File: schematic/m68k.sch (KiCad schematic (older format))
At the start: 45 parts, among them J1 Power, J2 CONN_01X03, J3 JTAG, J4 CONN_02X30, J5 I2C, J6 CONN_02X30, J7 CONN_01X02, J8 CONN_02X30, J9 CONN_01X03, SW1 SW_Push_Dual, U1 M68SEC000, U10 MCP23008, U2 AS6C8016, U3 LM1084IT-3.3/NOPB, U4 AT28BV64, U5 AT28BV64, U6 XC9572XL-VQ44, U7 MCP23017, U8 XO91-16, U9 XO91-50

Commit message: corrected footprints
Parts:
- J1: symbol Conn_01X04 -> CONN_01X04
- J2, J5, J9: symbol Conn_01X03 -> CONN_01X03
- J3: symbol Conn_01X06 -> CONN_01X06
- J4, J6, J8: symbol Conn_02X30 -> CONN_02X30
- J7: footprint Pin_Headers:Pin_Header_Straight_1x02 -> Pin_Headers:Pin_Header_Straight_1x02_Pitch2.54mm; symbol Conn_01X02 -> CONN_01X02
- U4, U5, U7: footprint SMD_Packages:SOIC-28 -> Housings_SOIC:SOIC-28W_7.5x17.9mm_Pitch1.27mm
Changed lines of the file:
@@
 LIBS:switches
 LIBS:m68k-cache
-EELAYER 26 0
+EELAYER 25 0
 EELAYER END
 $Descr A3 16535 11693
@@
 CLK_50MHz
 $Comp
-L Conn_01X06 J3
+L CONN_01X06 J3
 U 1 1 59881DD2
 P 4850 6750
@@
 $EndComp
 $Comp
-L Conn_01X03 J2
+L CONN_01X03 J2
 U 1 1 59883D86
 P 6150 6850
@@
 F 0 "U4" H 8200 2600 60  0000 C CNN
 F 1 "AT28BV64" H 8000 1100 60  0000 C CNN
-F 2 "SMD_Packages:SOIC-28" H 7950 1250 60  0001 C CNN
+F 2 "Housings_SOIC:SOIC-28W_7.5x17.9mm_Pitch1.27mm" H 7950 1250 60  0001 C CNN
 F 3 "" H 7950 1250 60  0001 C CNN
 	1    8000 1900
@@
 F 0 "U5" H 8200 4400 60  0000 C CNN
 F 1 "AT28BV64" H 8000 2900 60  0000 C CNN
-F 2 "SMD_Packages:SOIC-28" H 7950 3050 60  0001 C CNN
+F 2 "Housings_SOIC:SOIC-28W_7.5x17.9mm_Pitch1.27mm" H 7950 3050 60  0001 C CNN
 F 3 "" H 7950 3050 60  0001 C CNN
 	1    8000 3700
@@
 $EndComp
 $Comp
-L Conn_01X04 J1
+L CONN_01X04 J1
 U 1 1 5989E226
 P 3850 6850
@@
 F 0 "U7" H 12900 6075 50  0000 R CNN
 F 1 "MCP23017" H 12900 6000 50  0000 R CNN
-F 2 "SMD_Packages:SOIC-28" H 13050 4100 50  0001 L CNN
+F 2 "Housings_SOIC:SOIC-28W_7.5x17.9mm_Pitch1.27mm" H 13050 4100 50  0001 L CNN
 F 3 "" H 13250 6050 50  0001 C CNN
 	1    13000 5050
@@
 NoConn ~ 3250 1400
 $Comp
-L Conn_01X03 J5
+L CONN_01X03 J5
 U 1 1 598BE077
 P 2750 6800
@@
 Connection ~ 1950 6800
 $Comp
-L Conn_02X30 J4
+L CONN_02X30 J4
 U 1 1 598BF124
 P 7600 8900
@@
 ~HALT
 $Comp
-L Conn_01X03 J9
+L CONN_01X03 J9
 U 1 1 599050EF
 P 12300 3050
@@
 ~RESET
 $Comp
-L Conn_01X02 J7
+L CONN_01X02 J7
 U 1 1 59934E94
 P 9550 1700
 F 0 "J7" H 9550 1850 50  0000 C CNN
 F 1 "CONN_01X02" V 9650 1700 50  0000 C CNN
-F 2 "Pin_Headers:Pin_Header_Straight_1x02" H 9550 1700 50  0001 C CNN
+F 2 "Pin_Headers:Pin_Header_Straight_1x02_Pitch2.54mm" H 9550 1700 50  0001 C CNN
 F 3 "" H 9550 1700 50  0001 C CNN
 	1    9550 1700
@@
 ~IPL2
 $Comp
-L Conn_02X30 J6
+L CONN_02X30 J6
 U 1 1 5997FD38
 P 8750 8900
@@
 ~IPL2
 $Comp
-L Conn_02X30 J8
+L CONN_02X30 J8
 U 1 1 5997FDC7
 P 9900 8900

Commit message: bla
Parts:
- U3: footprint TO_SOT_Packages_THT:TO-220_Vertical -> TO_SOT_Packages_THT:TO-220_Horizontal
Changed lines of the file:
@@
 LIBS:switches
 LIBS:m68k-cache
-EELAYER 25 0
+EELAYER 26 0
 EELAYER END
 $Descr A3 16535 11693
@@
 F 0 "U3" H 5100 4600 50  0000 C CNN
 F 1 "LM1084IT-3.3/NOPB" H 4600 5000 50  0000 L CNN
-F 2 "TO_SOT_Packages_THT:TO-220_Vertical" H 4900 4900 50  0001 C CIN
+F 2 "TO_SOT_Packages_THT:TO-220_Horizontal" H 4900 4900 50  0001 C CIN
 F 3 "" H 4900 4800 50  0001 C CNN
 	1    4900 4800

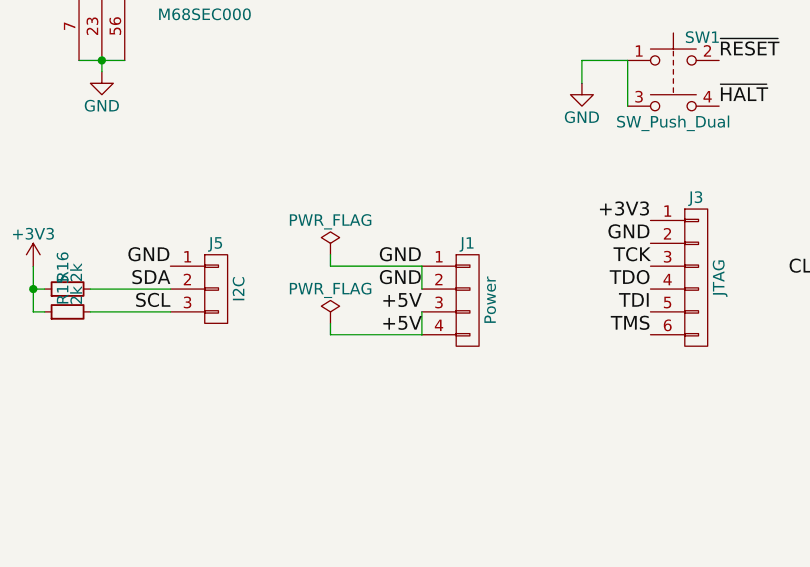
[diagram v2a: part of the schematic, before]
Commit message: bla
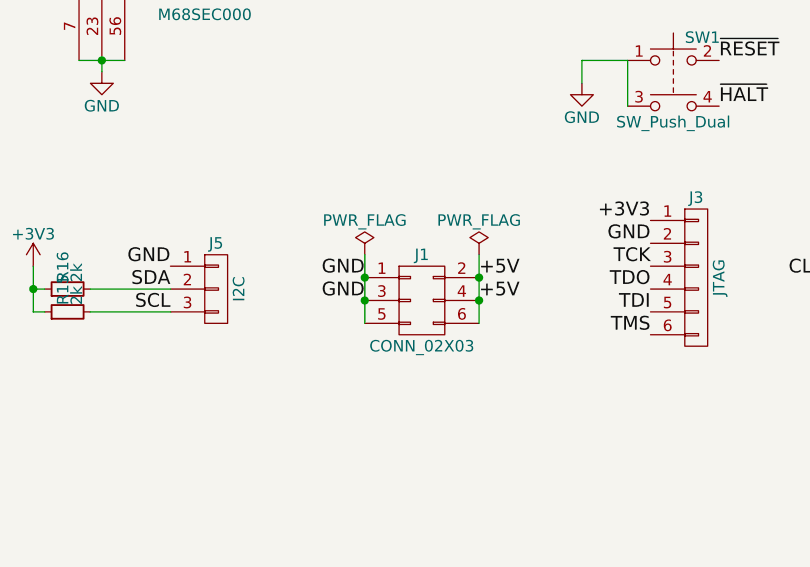
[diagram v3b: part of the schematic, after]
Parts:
- removed J1: Power, Pin_Headers:Pin_Header_Straight_1x04_Pitch2.54mm, symbol CONN_01X04
- added J1: CONN_02X03, Connectors:IDC_Header_Straight_6pins, symbol CONN_02X03
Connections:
- net +5V: now also J1.2 (P2), J1.4 (P4), J1.6 (P6)
- net GND: now also J1.1 (P1), J1.3 (P3), J1.5 (P5)
